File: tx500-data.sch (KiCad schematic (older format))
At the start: 51 parts, among them J1 USB_B_Micro, J2 CAT, J3 REM/DATA, J4 USB_A, U1 TUSB2036, U2 FT232RL, U3 HS-100B, U4 TPS76333, U5 TPS2044D, U6 SN75240, U7 SN75240, Y1 6MHz

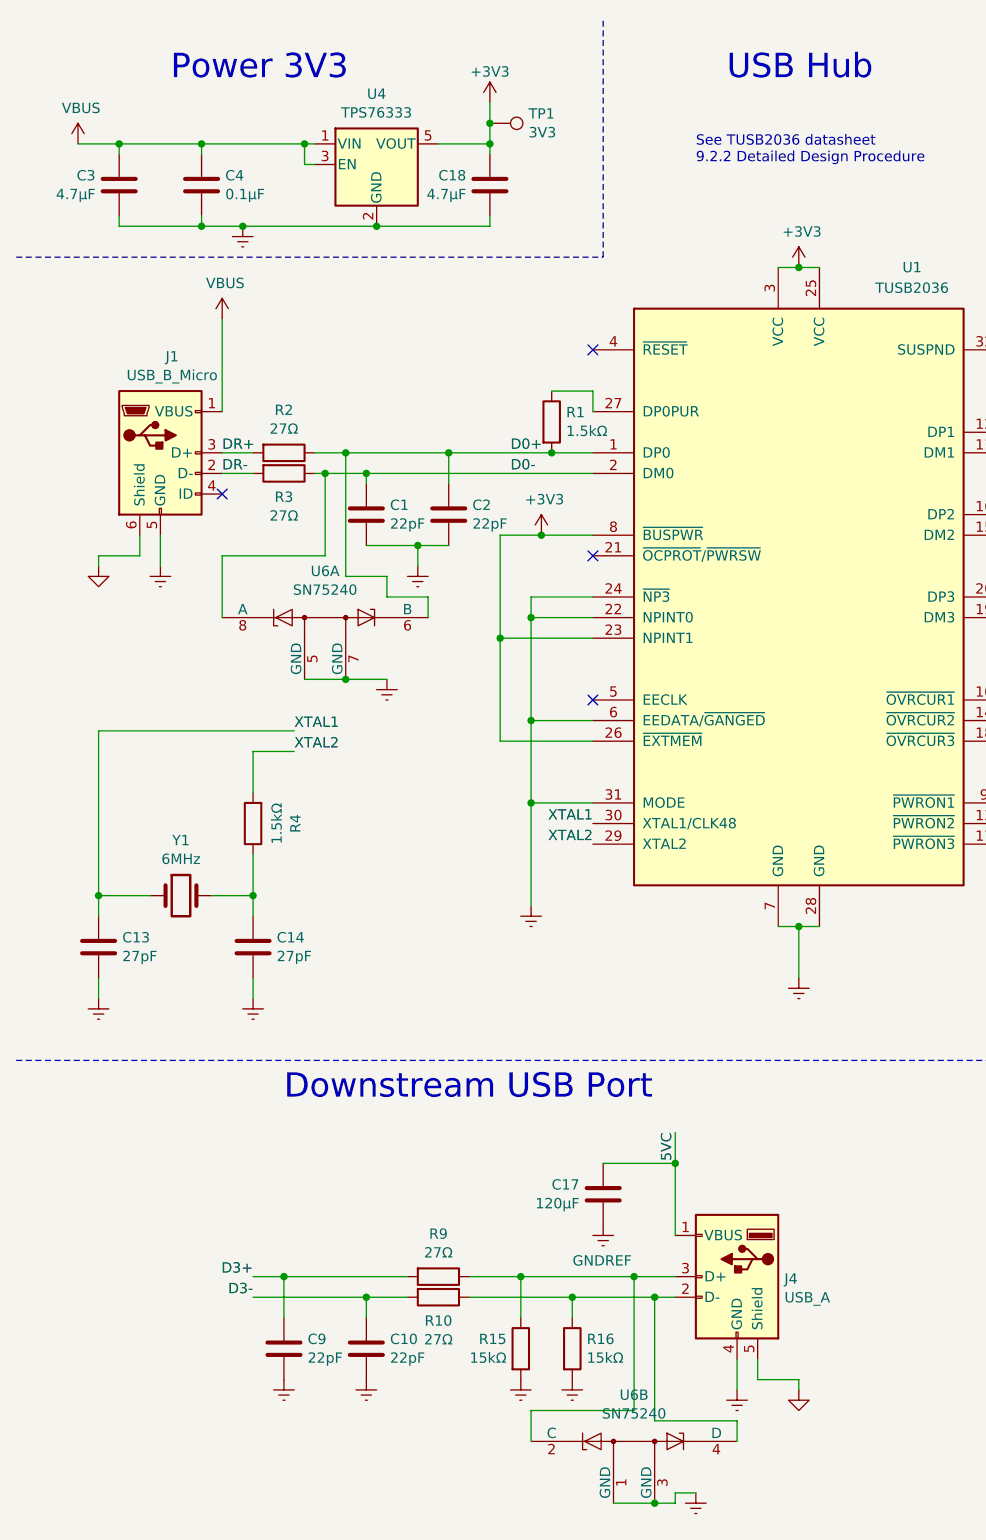
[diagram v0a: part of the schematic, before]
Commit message: Add 3D models, and various cleanup
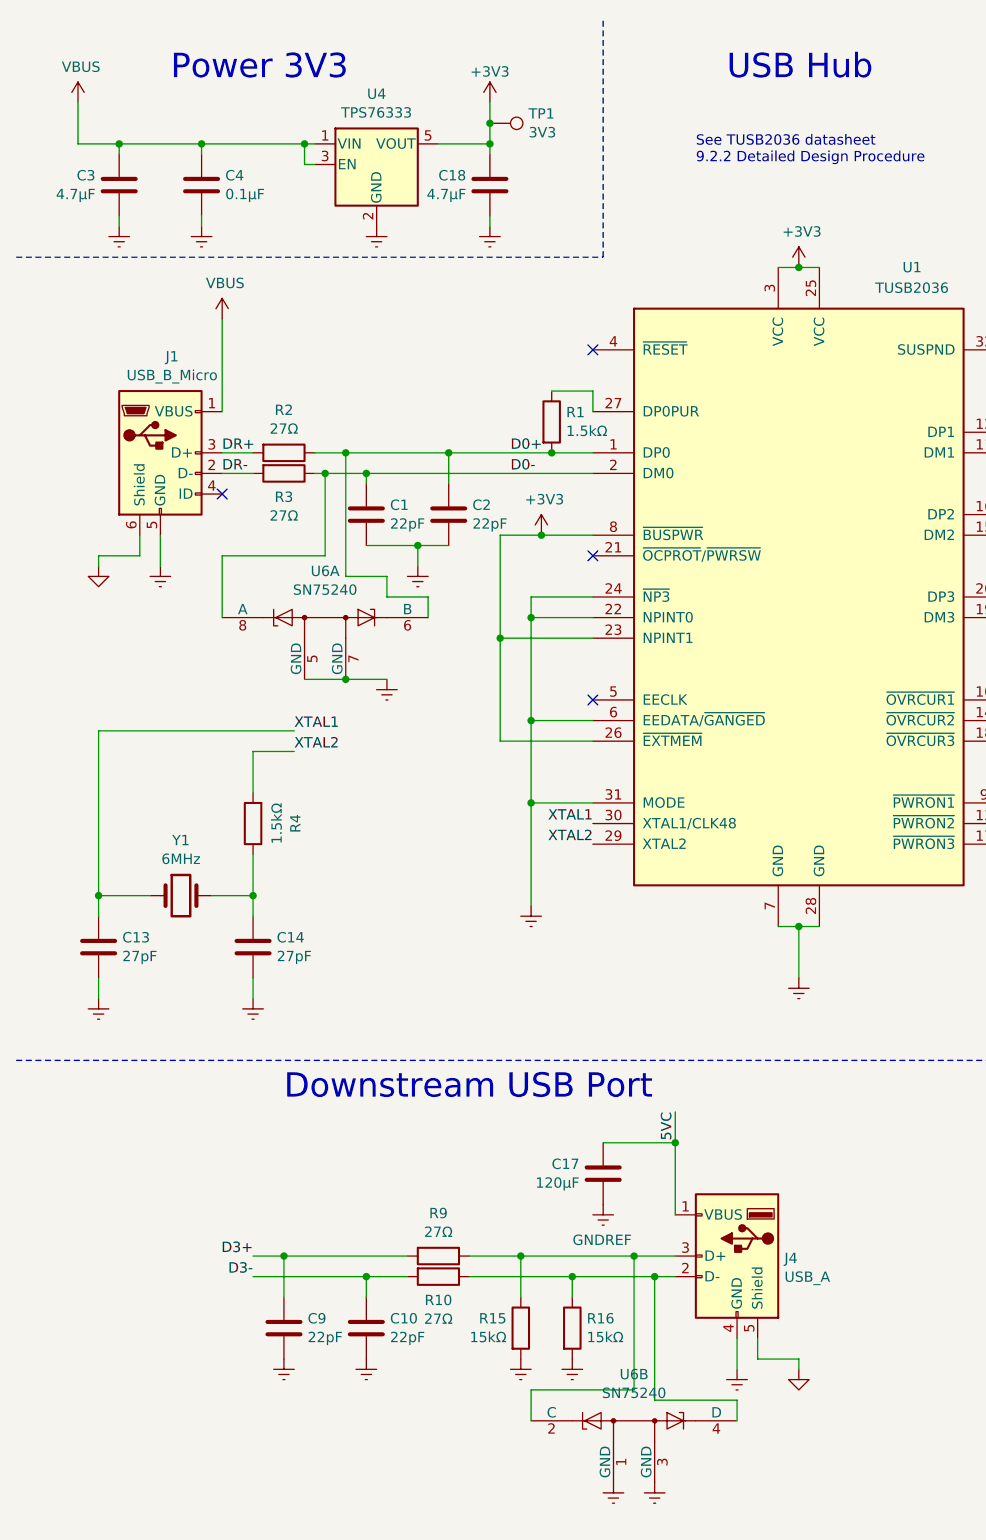
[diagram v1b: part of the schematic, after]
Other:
- moved on the sheet: C10, C17, C9, J4, R10, R15, R16, R9, U6B
